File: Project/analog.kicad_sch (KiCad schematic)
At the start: 22 parts, among them U4 74HC4051, U5 OPA350, U6 74HC4051

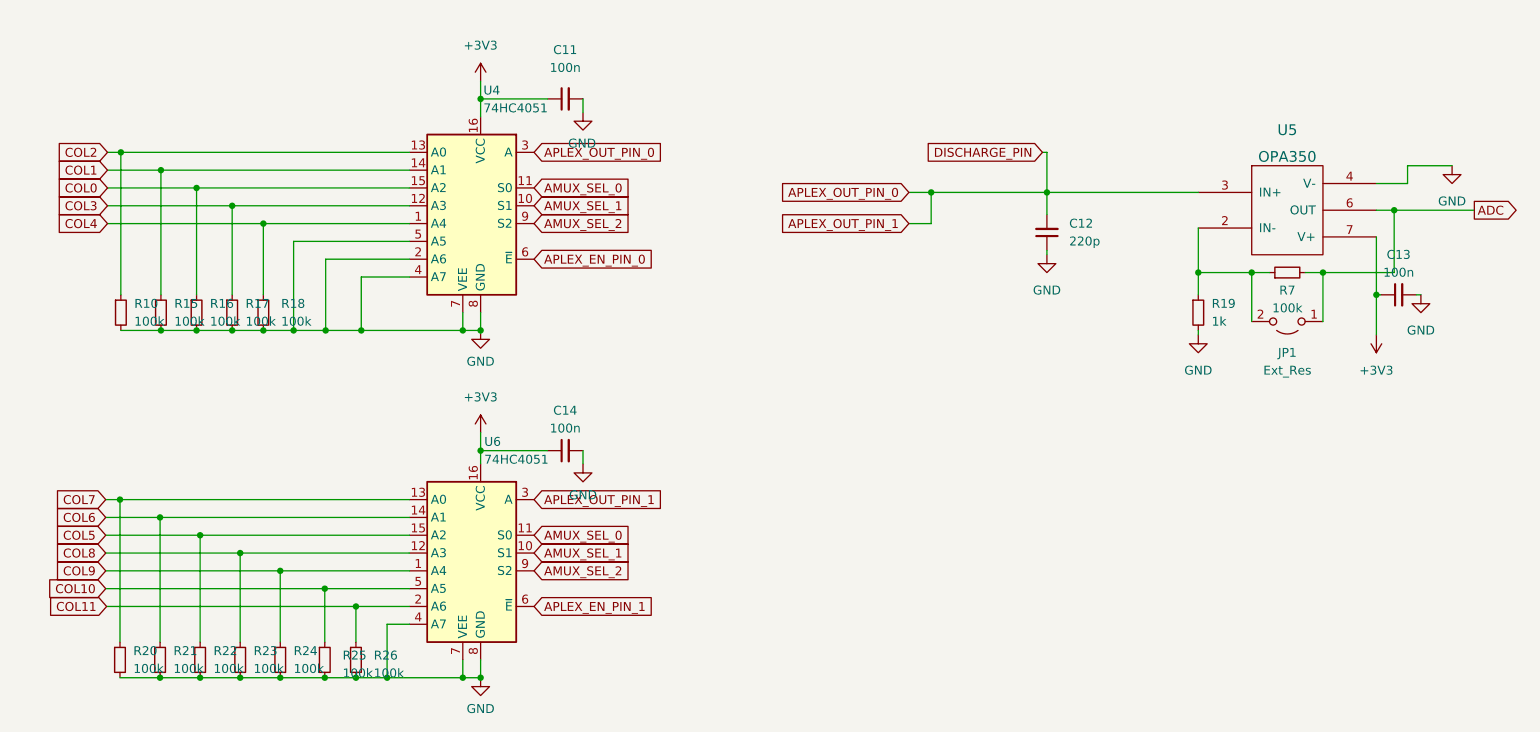
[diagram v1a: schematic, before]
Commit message: backup
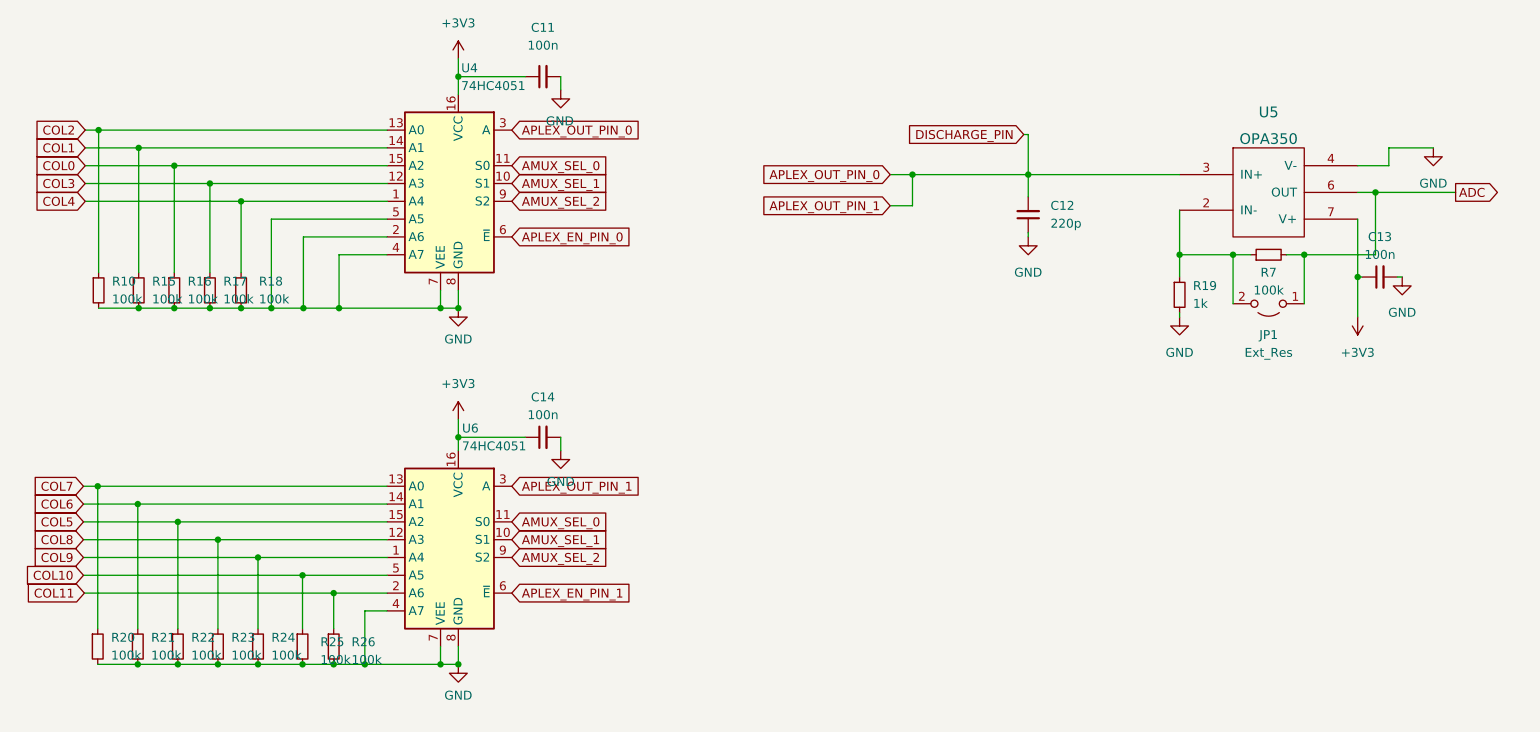
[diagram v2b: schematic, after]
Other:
- moved on the sheet: C11, C12, C13, C14, JP1, R10, R15, R16, R17, R18, R19, R20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
